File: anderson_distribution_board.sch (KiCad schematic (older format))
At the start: 5 parts, among them J1 Anderson_two_redblack, J2 Anderson_two_redblack, J3 Anderson_two_redblack, J4 Anderson_two_redblack, J5 Anderson_two_redblack

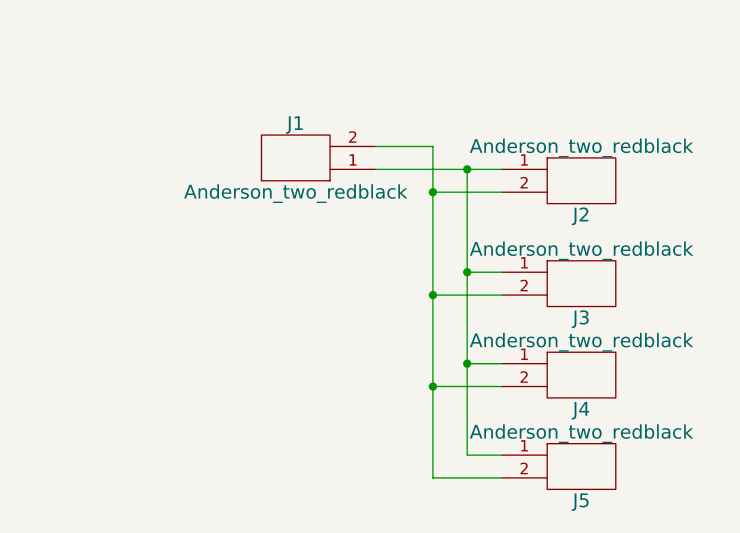
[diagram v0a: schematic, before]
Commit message: Polish and add gerbers
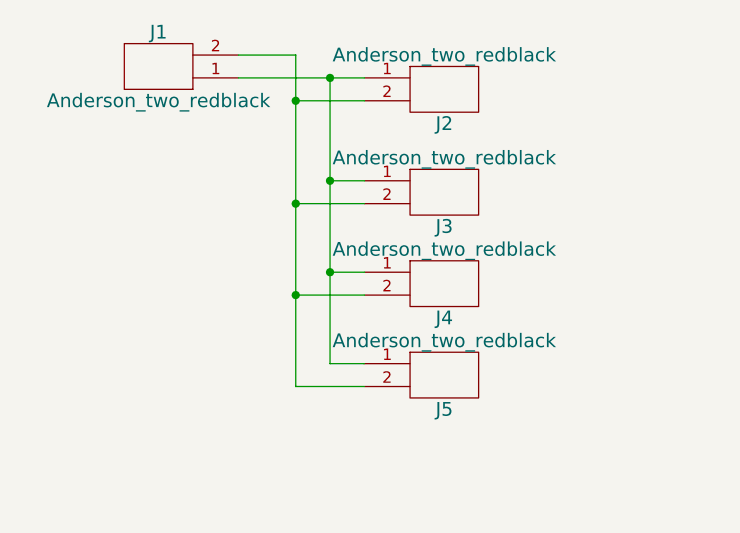
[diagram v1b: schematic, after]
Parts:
- J1: footprint (none) -> homebrew:Anderson_1337G3_right_angle_bottom_two
- J2, J3, J4, J5: footprint (none) -> homebrew:Anderson_1337G3_straight_two
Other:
- moved on the sheet: J1, J2, J3, J4, J5
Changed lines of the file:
@@
 EELAYER 25 0
 EELAYER END
-$Descr A4 11693 8268
+$Descr User 7874 5906
 encoding utf-8
 Sheet 1 1
@@
 L Anderson_two_redblack J1
 U 1 1 5B233648
-P 2150 2050
-F 0 "J1" H 2150 1900 60  0000 C CNN
-F 1 "Anderson_two_redblack" H 2150 2200 60  0000 C CNN
-F 2 "" H 2100 1900 60  0001 C CNN
-F 3 "" H 2100 1900 60  0001 C CNN
-	1    2150 2050
+P 1550 1650
+F 0 "J1" H 1550 1500 60  0000 C CNN
+F 1 "Anderson_two_redblack" H 1550 1800 60  0000 C CNN
+F 2 "homebrew:Anderson_1337G3_right_angle_bottom_two" H 1500 1500 60  0001 C CNN
+F 3 "" H 1500 1500 60  0001 C CNN
+	1    1550 1650
 	-1   0    0    1
 $EndComp
@@
 L Anderson_two_redblack J2
 U 1 1 5B2336FF
-P 3400 2150
-F 0 "J2" H 3400 2000 60  0000 C CNN
-F 1 "Anderson_two_redblack" H 3400 2300 60  0000 C CNN
-F 2 "" H 3350 2000 60  0001 C CNN
-F 3 "" H 3350 2000 60  0001 C CNN
-	1    3400 2150
+P 2800 1750
+F 0 "J2" H 2800 1600 60  0000 C CNN
+F 1 "Anderson_two_redblack" H 2800 1900 60  0000 C CNN
+F 2 "homebrew:Anderson_1337G3_straight_two" H 2750 1600 60  0001 C CNN
+F 3 "" H 2750 1600 60  0001 C CNN
+	1    2800 1750
 	1    0    0    -1
 $EndComp
@@
 L Anderson_two_redblack J3
 U 1 1 5B2337AB
-P 3400 2600
-F 0 "J3" H 3400 2450 60  0000 C CNN
-F 1 "Anderson_two_redblack" H 3400 2750 60  0000 C CNN
-F 2 "" H 3350 2450 60  0001 C CNN
-F 3 "" H 3350 2450 60  0001 C CNN
-	1    3400 2600
+P 2800 2200
+F 0 "J3" H 2800 2050 60  0000 C CNN
+F 1 "Anderson_two_redblack" H 2800 2350 60  0000 C CNN
+F 2 "homebrew:Anderson_1337G3_straight_two" H 2750 2050 60  0001 C CNN
+F 3 "" H 2750 2050 60  0001 C CNN
+	1    2800 2200
 	1    0    0    -1
 $EndComp
@@
 L Anderson_two_redblack J5
 U 1 1 5B2337D4
-P 3400 3400
-F 0 "J5" H 3400 3250 60  0000 C CNN
-F 1 "Anderson_two_redblack" H 3400 3550 60  0000 C CNN
-F 2 "" H 3350 3250 60  0001 C CNN
-F 3 "" H 3350 3250 60  0001 C CNN
-	1    3400 3400
+P 2800 3000
+F 0 "J5" H 2800 2850 60  0000 C CNN
+F 1 "Anderson_two_redblack" H 2800 3150 60  0000 C CNN
+F 2 "homebrew:Anderson_1337G3_straight_two" H 2750 2850 60  0001 C CNN
+F 3 "" H 2750 2850 60  0001 C CNN
+	1    2800 3000
 	1    0    0    -1
 $EndComp
 Wire Wire Line
-	2500 2000 2750 2000
+	1900 1600 2150 1600
 Wire Wire Line
-	2750 2000 2750 3450
+	2150 1600 2150 3050
 Wire Wire Line
-	2750 3450 3050 3450
+	2150 3050 2450 3050
 Wire Wire Line
-	3050 2650 2750 2650
-Connection ~ 2750 2650
+	2450 2250 2150 2250
+Connection ~ 2150 2250
 Wire Wire Line
-	3050 2200 2750 2200
-Connection ~ 2750 2200
+	2450 1800 2150 1800
+Connection ~ 2150 1800
 Wire Wire Line
-	2500 2100 3050 2100
+	1900 1700 2450 1700
 Wire Wire Line
-	2900 2100 2900 3350
+	2300 1700 2300 2950
 Wire Wire Line
-	2900 2550 3050 2550
-Connection ~ 2900 2100
+	2300 2150 2450 2150
+Connection ~ 2300 1700
 Wire Wire Line
-	2900 3350 3050 3350
-Connection ~ 2900 2550
+	2300 2950 2450 2950
+Connection ~ 2300 2150
 $Comp
 L Anderson_two_redblack J4
 U 1 1 5B2338F7
-P 3400 3000
-F 0 "J4" H 3400 2850 60  0000 C CNN
-F 1 "Anderson_two_redblack" H 3400 3150 60  0000 C CNN
-F 2 "" H 3350 2850 60  0001 C CNN
-F 3 "" H 3350 2850 60  0001 C CNN
-	1    3400 3000
+P 2800 2600
+F 0 "J4" H 2800 2450 60  0000 C CNN
+F 1 "Anderson_two_redblack" H 2800 2750 60  0000 C CNN
+F 2 "homebrew:Anderson_1337G3_straight_two" H 2750 2450 60  0001 C CNN
+F 3 "" H 2750 2450 60  0001 C CNN
+	1    2800 2600
 	1    0    0    -1
 $EndComp
 Wire Wire Line
-	2900 2950 3050 2950
+	2300 2550 2450 2550
 Wire Wire Line
-	2750 3050 3050 3050
-Connection ~ 2750 3050
-Connection ~ 2900 2950
+	2150 2650 2450 2650
+Connection ~ 2150 2650
+Connection ~ 2300 2550
 $EndSCHEMATC
